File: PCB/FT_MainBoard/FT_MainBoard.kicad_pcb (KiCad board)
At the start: 2 copper layers, 110 x 75 mm, 71 parts, among them CON1 Conn_01x02_Pin, CON3 Conn_01x04_Pin, CON4 Conn_01x02_Pin, CON5 Conn_01x04_Pin, CON6 AVR-ISP-6, IC1 ATmega328PB-AU, IC2 FT231XS-R, IC3 74HC3G14DP,125, IC4 L78M05ABDT-TR, Q1 PMBT3904,215, Q2 PMBT3904,215, SW1 SW_Push, SW2 SW_Push, SW3 SW_Push, SW4 SW_Push, SW5 SW_SPST

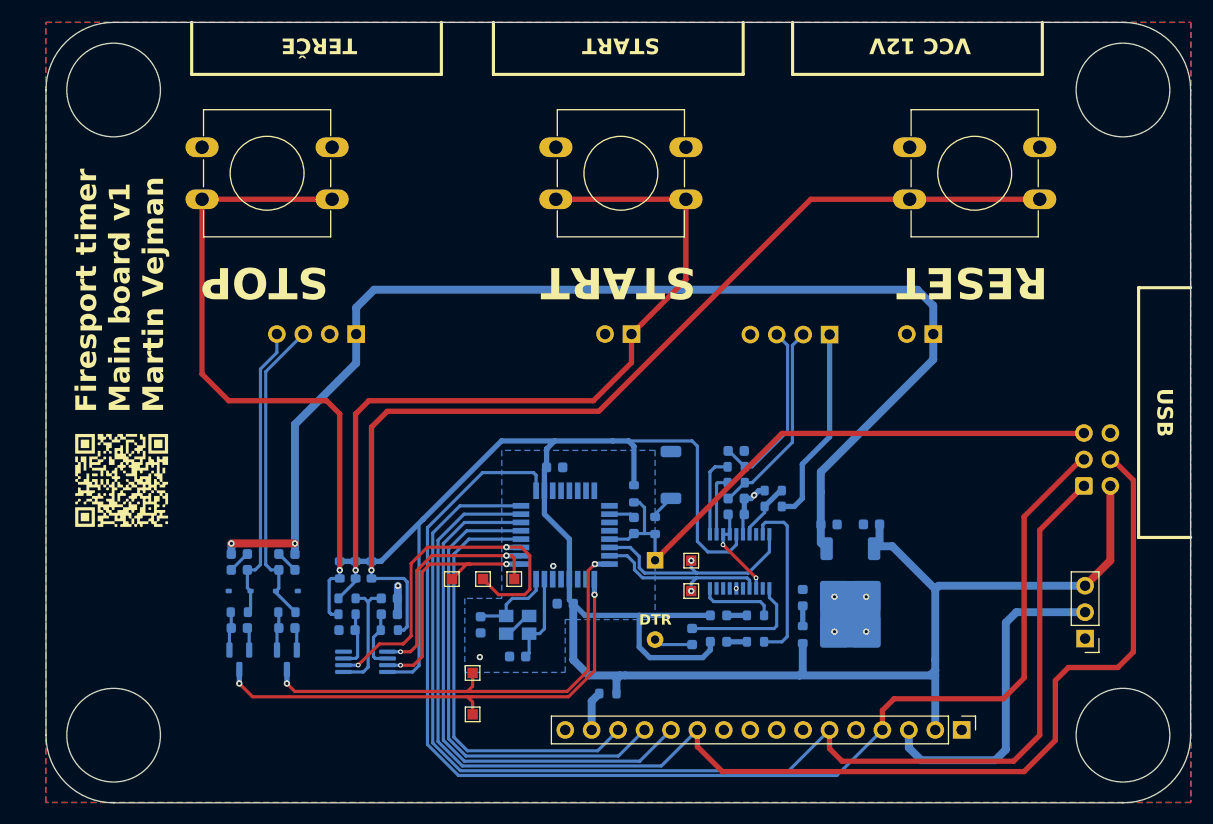
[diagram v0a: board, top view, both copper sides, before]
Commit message: panelization
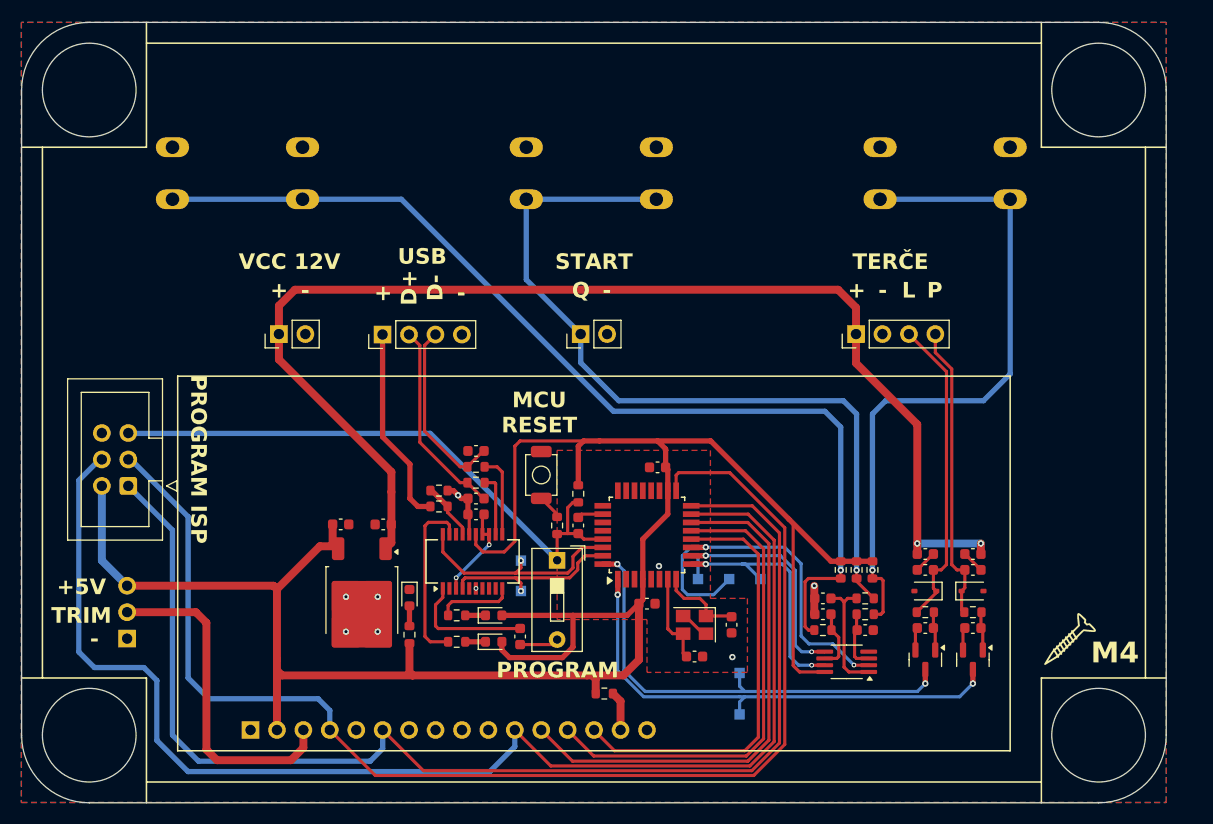
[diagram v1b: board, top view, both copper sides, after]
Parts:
- C1, C10, C11, C14, C15, C16, C17, C18, C2, C3, C4, C5, C6, C7, C8, C9, CON1, CON3, CON4, CON5, CON6, D1, D2, G***, IC1, IC2, IC3, IC4, LED1, LED2, LED3, OSC1, Q1, Q2, R1, R10, R11, R12, R13, R14, R15, R16, R17, R18, R19, R2, R20, R21, R22, R3, R4, R5, R6, R7, R8, R9, SW4, SW5: moved to F.Cu
- G***, HDR1, L, R, RESET, RV1, RX, START, STOP, SW1, SW2, SW3, TX: moved to B.Cu
- moved G*** 93.2 mm to (150.4, 94.0), turned to 180 degrees
- moved RV1 92.1 mm to (57.8, 109.2), turned to 0 degrees
- moved CON6 91.8 mm to (57.9, 94.5), turned to 180 degrees
- moved G*** 89.2 mm to (148.4, 109.2), turned to 0 degrees
- moved SW2 77.7 mm to (142.7, 62.0), turned to 180 degrees
- moved C15 70.5 mm to (139.1, 108.2), turned to 180 degrees
- moved Q2 70.5 mm to (139.1, 111.3)
- moved R13 70.5 mm to (139.1, 102.6), turned to 0 degrees
- moved R14 70.5 mm to (139.1, 101.1), turned to 0 degrees
- moved R17 70.5 mm to (139.1, 106.7), turned to 180 degrees
- moved D1 70.4 mm to (139.0, 104.6), turned to 0 degrees
- moved HDR1 68.3 mm to (69.7, 118.0)
- moved C14 61.4 mm to (134.5, 108.2), turned to 180 degrees
- moved D2 61.4 mm to (134.5, 104.6), turned to 180 degrees
- moved Q1 61.4 mm to (134.5, 111.3)
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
